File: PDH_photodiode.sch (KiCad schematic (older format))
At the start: 34 parts, among them J1 ±5V-Supply, J2 AC Out, J3 DC Out, U1 LT3032, U2 LTC6269-10

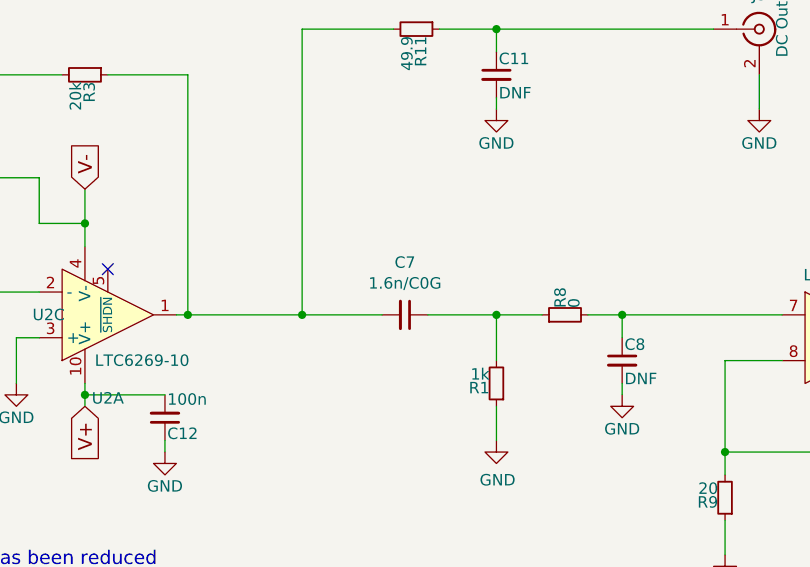
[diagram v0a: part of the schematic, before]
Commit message: Update BOM and gerber files
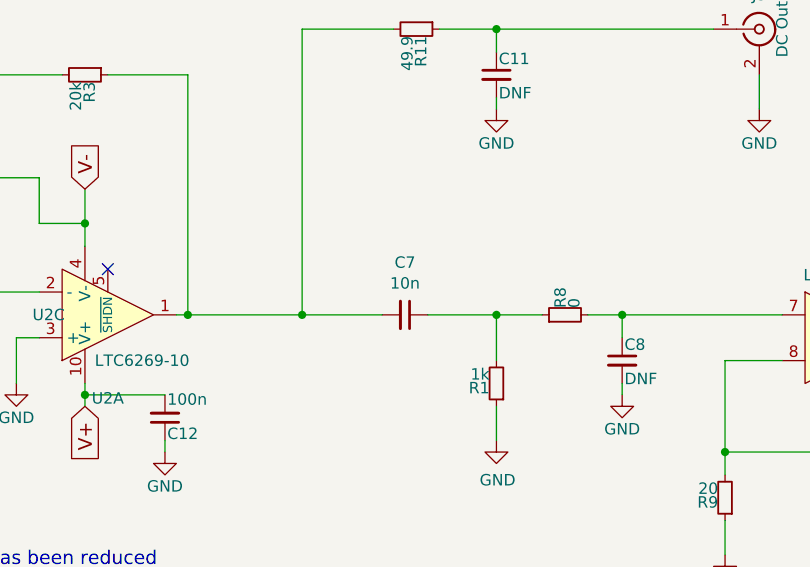
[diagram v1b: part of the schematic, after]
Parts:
- C1, C2, C5, C6: PN GMK325BJ106MN-T -> UMR325AC7106MM-P
- C7: value 1.6n/C0G -> 10n; MFN (none) -> Murata Electronics; PN (none) -> GRM1885C1H103JA01D
- D1: Config (none) -> DNF
- J2: Config DNF -> (none)
- R1: MFN Susumu -> Yageo; PN (none) -> RT0603DRE071KL
- R10: PN (none) -> RR0816P-181-D
- R2, R7: MFN (none) -> Susumu; PN (none) -> RR0816P-1053-D-03D
- R3: PN (none) -> RR0816P-203-D
- R5, R6: MFN (none) -> Susumu; PN (none) -> RR0816P-104-D
- R8: MFN Susumu -> Vishay/Beyschlag; PN (none) -> MCT06030Z0000ZP500
- R9: PN (none) -> RR0816Q-200-D
- U1: MFN (none) -> Analog Devices; PN (none) -> LT3032EDE#PBF
- U2: MFN (none) -> Analog Devices; PN (none) -> LTC6269HDD-10#PBF
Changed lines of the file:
@@
 F 3 "" H 4000 4750 50  0001 C CNN
 F 4 "Taiyo Yuden" H 4000 4750 60  0001 C CNN "MFN"
-F 5 "GMK325BJ106MN-T" H 4000 4750 50  0001 C CNN "PN"
+F 5 "UMR325AC7106MM-P" H 4000 4750 50  0001 C CNN "PN"
 	1    4000 4750
 	1    0    0    -1
@@
 F 3 "" H 4000 5450 50  0001 C CNN
 F 4 "Taiyo Yuden" H 4000 5450 60  0001 C CNN "MFN"
-F 5 "GMK325BJ106MN-T" H 4000 5450 50  0001 C CNN "PN"
+F 5 "UMR325AC7106MM-P" H 4000 5450 50  0001 C CNN "PN"
 	1    4000 5450
 	1    0    0    -1
@@
 F 3 "" H 4500 1400 50  0001 C CNN
 F 4 "Susumu" H 4500 1400 60  0001 C CNN "MFN"
-F 5 "" H 4500 1400 50  0001 C CNN "PN"
+F 5 "RR0816P-203-D" H 4500 1400 50  0001 C CNN "PN"
 	1    4500 1400
 	0    1    1    0
@@
 F 3 "" H 6950 4900 50  0001 C CNN
 F 4 "Taiyo Yuden" H 6950 4900 60  0001 C CNN "MFN"
-F 5 "GMK325BJ106MN-T" H 6950 4900 50  0001 C CNN "PN"
+F 5 "UMR325AC7106MM-P" H 6950 4900 50  0001 C CNN "PN"
 	1    6950 4900
 	1    0    0    -1
@@
 F 3 "" H 6950 5400 50  0001 C CNN
 F 4 "Taiyo Yuden" H 6950 5400 60  0001 C CNN "MFN"
-F 5 "GMK325BJ106MN-T" H 6950 5400 50  0001 C CNN "PN"
+F 5 "UMR325AC7106MM-P" H 6950 5400 50  0001 C CNN "PN"
 	1    6950 5400
 	1    0    0    -1
@@
 F 2 "Package_DFN_QFN:Linear_DE14MA" H 5350 5025 50  0001 C CNN
 F 3 "https://www.analog.com/media/en/technical-documentation/data-sheets/3032ff.pdf" H 5350 4700 50  0001 C CNN
+F 4 "Analog Devices" H 5350 4700 50  0001 C CNN "MFN"
+F 5 "LT3032EDE#PBF" H 5350 4700 50  0001 C CNN "PN"
 	1    5350 4700
 	1    0    0    -1
@@
 F 2 "Package_DFN_QFN:Linear_DE14MA" H 5350 5825 50  0001 C CNN
 F 3 "https://www.analog.com/media/en/technical-documentation/data-sheets/3032ff.pdf" H 5350 5500 50  0001 C CNN
+F 4 "Analog Devices" H 5350 5500 50  0001 C CNN "MFN"
+F 5 "LT3032EDE#PBF" H 5350 5500 50  0001 C CNN "PN"
 	2    5350 5500
 	1    0    0    1
@@
 F 2 "Resistor_SMD:R_0603_1608Metric" H 6450 4700 50  0001 C CNN
 F 3 "~" H 6450 4700 50  0001 C CNN
+F 4 "Susumu" H 6450 4700 50  0001 C CNN "MFN"
+F 5 "RR0816P-1053-D-03D" H 6450 4700 50  0001 C CNN "PN"
 	1    6450 4700
 	1    0    0    -1
@@
 F 2 "Resistor_SMD:R_0603_1608Metric" H 6450 5000 50  0001 C CNN
 F 3 "~" H 6450 5000 50  0001 C CNN
+F 4 "Susumu" H 6450 5000 50  0001 C CNN "MFN"
+F 5 "RR0816P-104-D" H 6450 5000 50  0001 C CNN "PN"
 	1    6450 5000
 	1    0    0    -1
@@
 F 2 "Resistor_SMD:R_0603_1608Metric" H 6450 5500 50  0001 C CNN
 F 3 "~" H 6450 5500 50  0001 C CNN
+F 4 "Susumu" H 6450 5500 50  0001 C CNN "MFN"
+F 5 "RR0816P-1053-D-03D" H 6450 5500 50  0001 C CNN "PN"
 	1    6450 5500
 	1    0    0    -1
@@
 F 2 "Resistor_SMD:R_0603_1608Metric" H 6450 5200 50  0001 C CNN
 F 3 "~" H 6450 5200 50  0001 C CNN
+F 4 "Susumu" H 6450 5200 50  0001 C CNN "MFN"
+F 5 "RR0816P-104-D" H 6450 5200 50  0001 C CNN "PN"
 	1    6450 5200
 	1    0    0    -1
@@
 F 4 "Hamamatsu" V 3050 2650 50  0001 C CNN "MFN"
 F 5 "S9055-01" V 3050 2650 50  0001 C CNN "PN"
+F 6 "DNF" V 3050 2650 50  0001 C CNN "Config"
 	1    3050 2650
 	0    1    1    0
@@
 F 2 "Package_DFN_QFN:DFN-10-1EP_3x3mm_P0.5mm_EP1.65x2.38mm" H 4600 2050 50  0001 C CNN
 F 3 "" H 4600 2450 50  0001 C CNN
+F 4 "Analog Devices" H 4600 2450 50  0001 C CNN "MFN"
+F 5 "LTC6269HDD-10#PBF" H 4600 2450 50  0001 C CNN "PN"
 	1    4600 2450
 	1    0    0    1
@@
 F 2 "Package_DFN_QFN:DFN-10-1EP_3x3mm_P0.5mm_EP1.65x2.38mm" H 7850 2150 50  0001 C CNN
 F 3 "" H 7850 2550 50  0001 C CNN
+F 4 "Analog Devices" H 7850 2550 50  0001 C CNN "MFN"
+F 5 "LTC6269HDD-10#PBF" H 7850 2550 50  0001 C CNN "PN"
 	2    7850 2550
 	1    0    0    -1
@@
 P 5900 2450
 F 0 "C7" V 5671 2450 50  0000 C CNN
-F 1 "1.6n/C0G" V 5762 2450 50  0000 C CNN
+F 1 "10n" V 5762 2450 50  0000 C CNN
 F 2 "Capacitor_SMD:C_0603_1608Metric" H 5900 2450 50  0001 C CNN
 F 3 "~" H 5900 2450 50  0001 C CNN
+F 4 "Murata Electronics" V 5900 2450 50  0001 C CNN "MFN"
+F 5 "GRM1885C1H103JA01D" V 5900 2450 50  0001 C CNN "PN"
 	1    5900 2450
 	0    1    1    0
@@
 F 2 "Resistor_SMD:R_0603_1608Metric" H 6300 2750 50  0001 C CNN
 F 3 "" H 6300 2750 50  0001 C CNN
-F 4 "Susumu" H 6300 2750 60  0001 C CNN "MFN"
-F 5 "" H 6300 2750 50  0001 C CNN "PN"
+F 4 "Yageo" H 6300 2750 60  0001 C CNN "MFN"
+F 5 "RT0603DRE071KL" H 6300 2750 50  0001 C CNN "PN"
 	1    6300 2750
 	-1   0    0    1
@@
 F 3 "" H 7300 3250 50  0001 C CNN
 F 4 "Susumu" H 7300 3250 60  0001 C CNN "MFN"
-F 5 "" H 7300 3250 50  0001 C CNN "PN"
+F 5 "RR0816Q-200-D" H 7300 3250 50  0001 C CNN "PN"
 	1    7300 3250
 	-1   0    0    1
@@
 F 3 "" H 7800 3050 50  0001 C CNN
 F 4 "Susumu" H 7800 3050 60  0001 C CNN "MFN"
-F 5 "" H 7800 3050 50  0001 C CNN "PN"
+F 5 "RR0816P-181-D" H 7800 3050 50  0001 C CNN "PN"
 	1    7800 3050
 	0    -1   -1   0
@@
 F 2 "Resistor_SMD:R_0603_1608Metric" H 6600 2450 50  0001 C CNN
 F 3 "" H 6600 2450 50  0001 C CNN
-F 4 "Susumu" H 6600 2450 60  0001 C CNN "MFN"
-F 5 "" H 6600 2450 50  0001 C CNN "PN"
+F 4 "Vishay/Beyschlag" H 6600 2450 60  0001 C CNN "MFN"
+F 5 "MCT06030Z0000ZP500" H 6600 2450 50  0001 C CNN "PN"
 	1    6600 2450
 	0    -1   -1   0
@@
 F 4 "Amphenol" H 10400 2550 50  0001 C CNN "MFN"
 F 5 "901-143-6RFX" H 10400 2550 50  0001 C CNN "PN"
-F 6 "DNF" H 10400 2550 50  0001 C CNN "Config"
+F 6 "" H 10400 2550 50  0001 C CNN "Config"
 	1    10400 2550
 	1    0    0    -1
